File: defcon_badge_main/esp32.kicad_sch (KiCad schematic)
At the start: 20 parts, among them J1 USB_C_Receptacle, U3 ESP32-C5-WROOM-1U

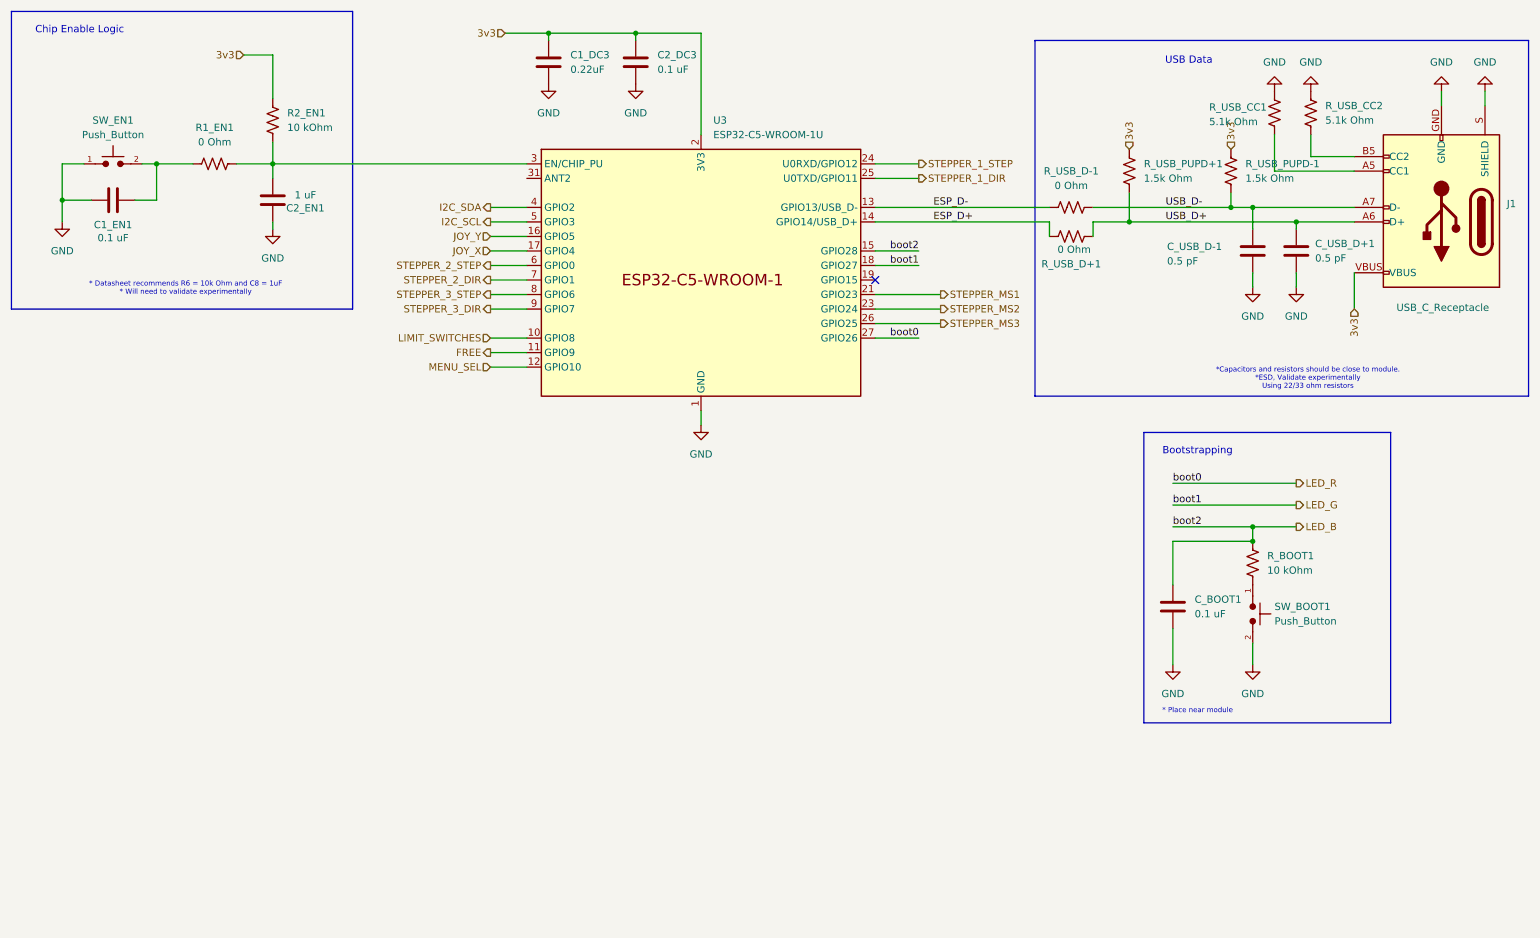
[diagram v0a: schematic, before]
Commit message: begin full layout
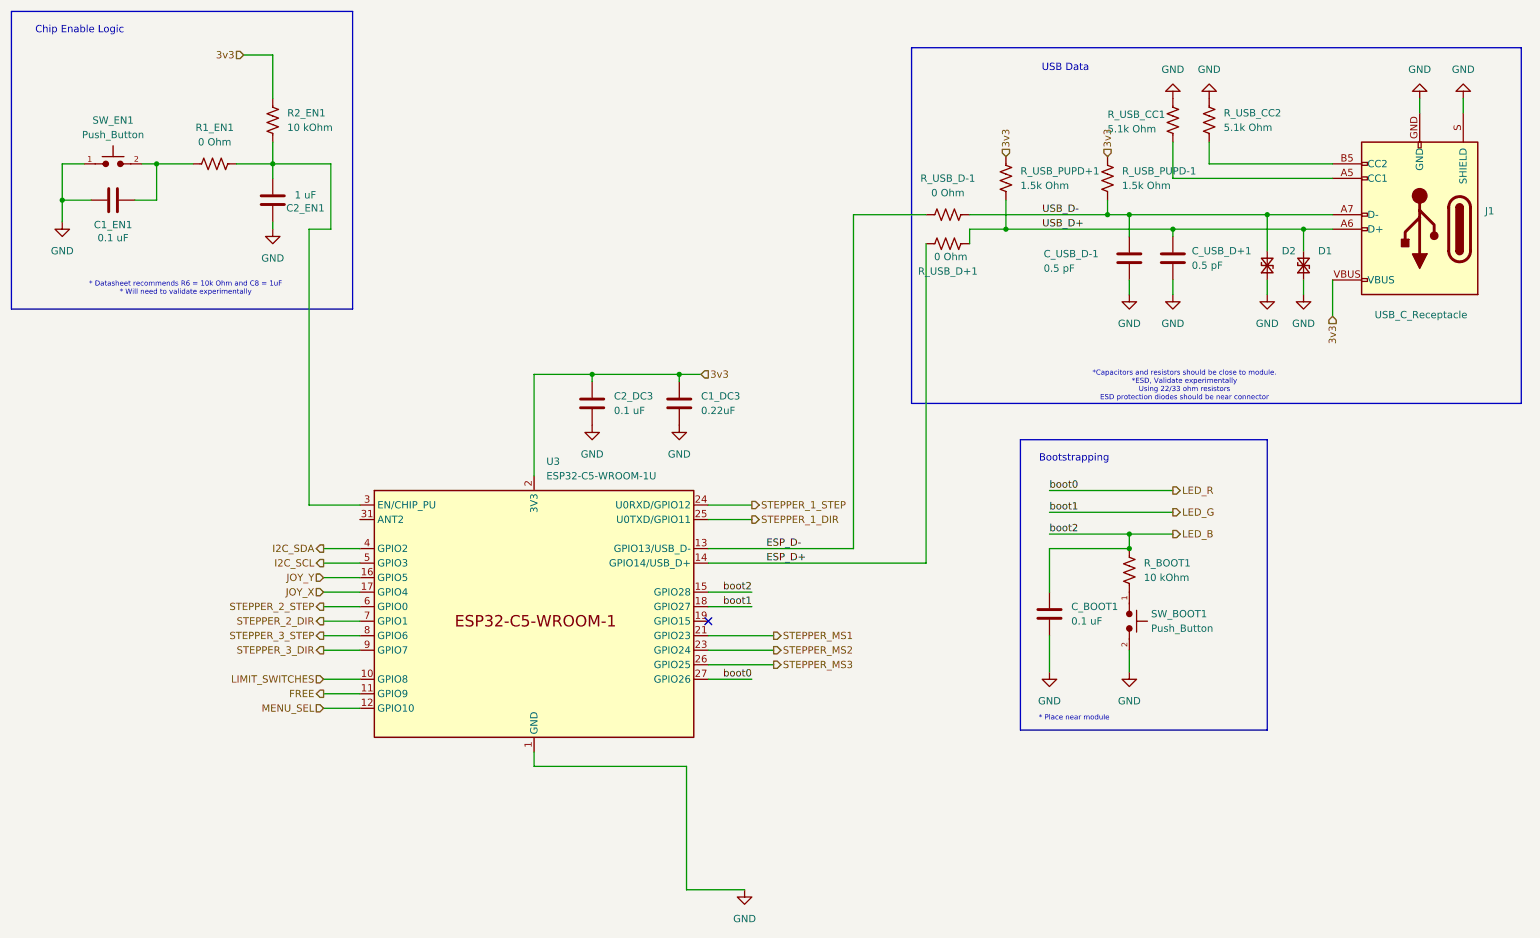
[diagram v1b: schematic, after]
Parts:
- added D1, D2: PESD0402, PCM_SparkFun-Capacitor:C_0402_1005Metric, symbol PCM_SparkFun-DiscreteSemi:D_TVS_0402_14V
- R_BOOT1: footprint PCM_SparkFun-Fuse:1206 -> PCM_SparkFun-Coil:0805
- R_USB_D+1, R_USB_D-1, R_USB_PUPD+1, R_USB_PUPD-1: footprint PCM_SparkFun-Coil:0805 -> Resistor_SMD:R_0402_1005Metric
- SW_BOOT1, SW_EN1: footprint Button_Switch_SMD:SW_SPST_PTS645 -> Button_Switch_SMD:SW_SPST_PTS810
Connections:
- net GND: now also D1.1 (A1), D2.1 (A1)
- net USB_D+: now also D1.2 (A2)
- net USB_D-: now also D2.2 (A2)
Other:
- note added: "*Capacitors and resistors should be close to module. *ESD, Validate experimentally Using 22/33 ohm resistors ESD protection diodes should be near connector"
- note removed: "*Capacitors and resistors should be close to module. *ESD, Validate experimentally Using 22/33 ohm resistors"
- moved on the sheet: C1_DC3, C2_DC3, C_BOOT1, C_USB_D+1, C_USB_D-1, J1, R_BOOT1, R_USB_CC1, R_USB_CC2, R_USB_D+1, R_USB_D-1, R_USB_PUPD+1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
